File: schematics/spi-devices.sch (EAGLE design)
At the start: 13 parts, among them J1 DM3AT-SF-PEJM5, X1 87758-1016, X2 87758-0216

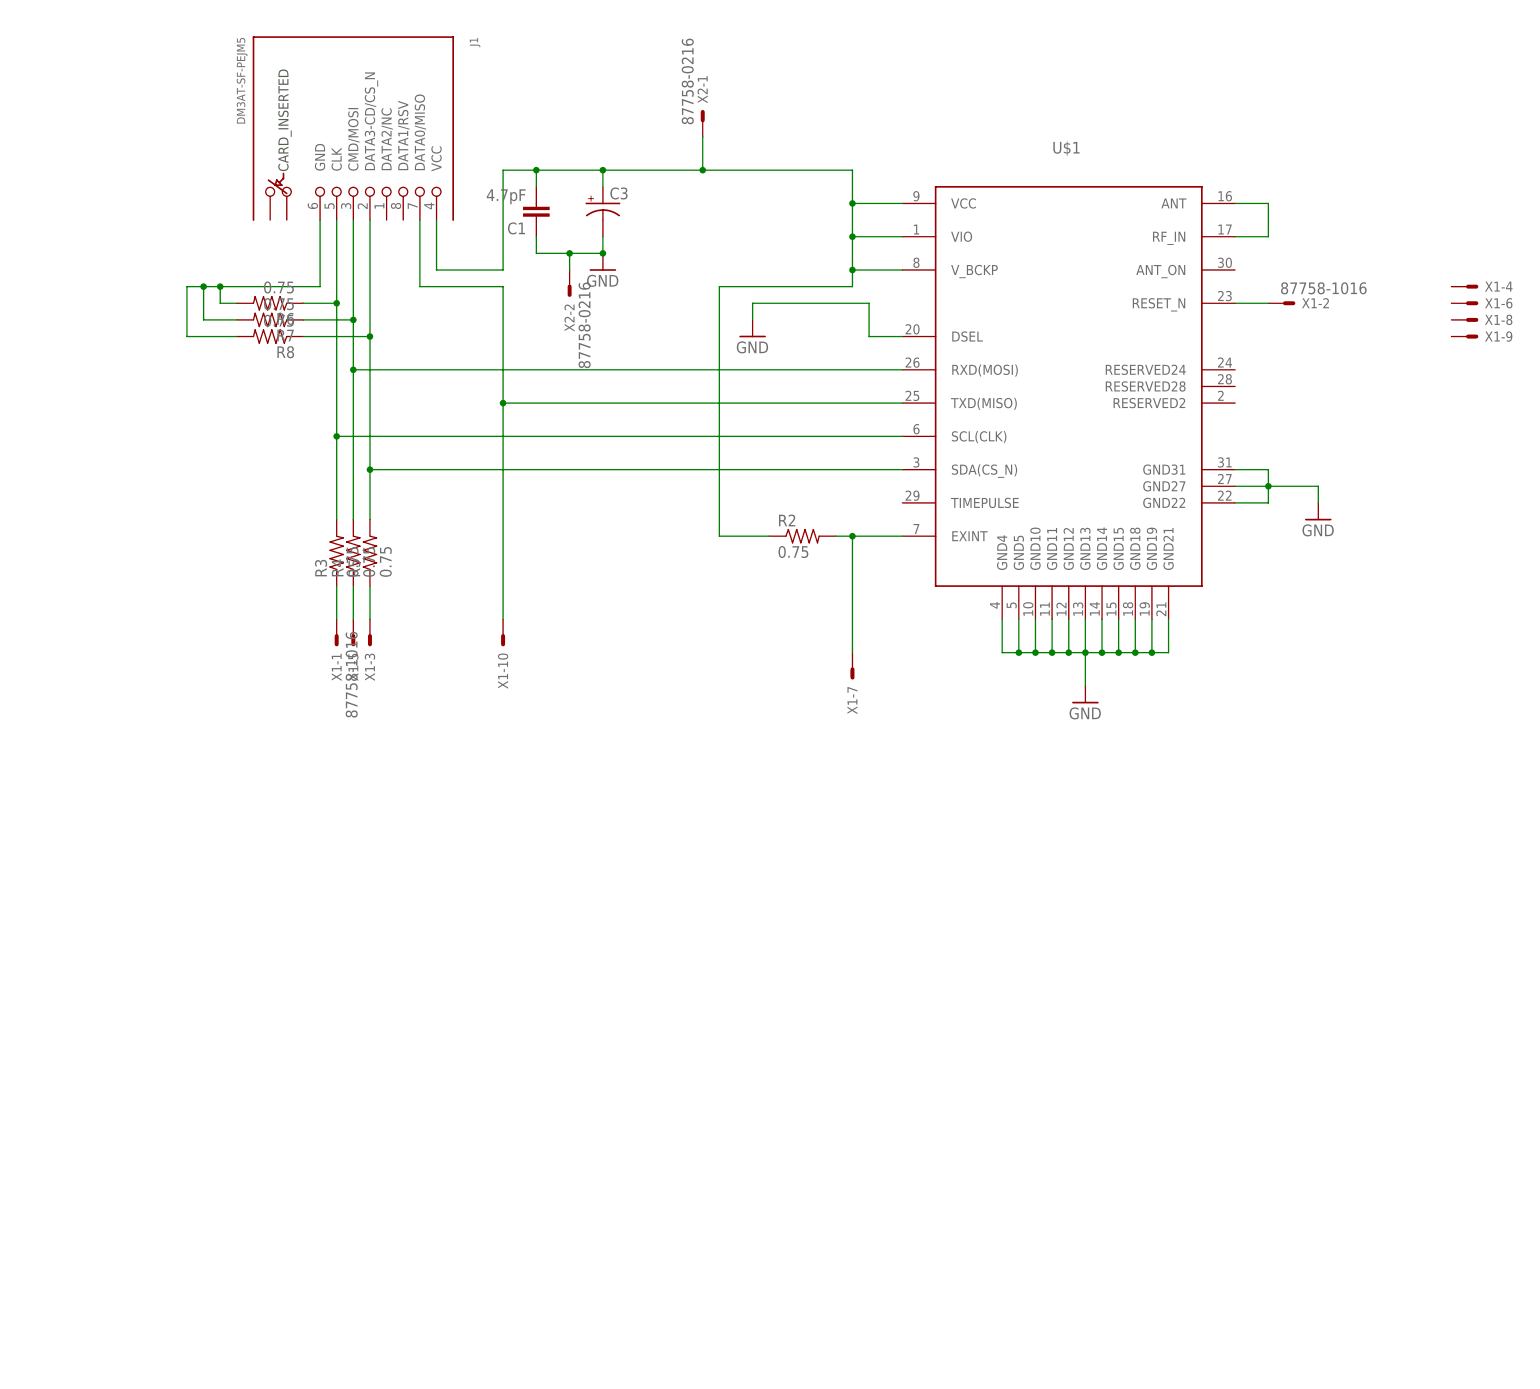
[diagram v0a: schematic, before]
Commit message: Платы, правки, накопленные изменения
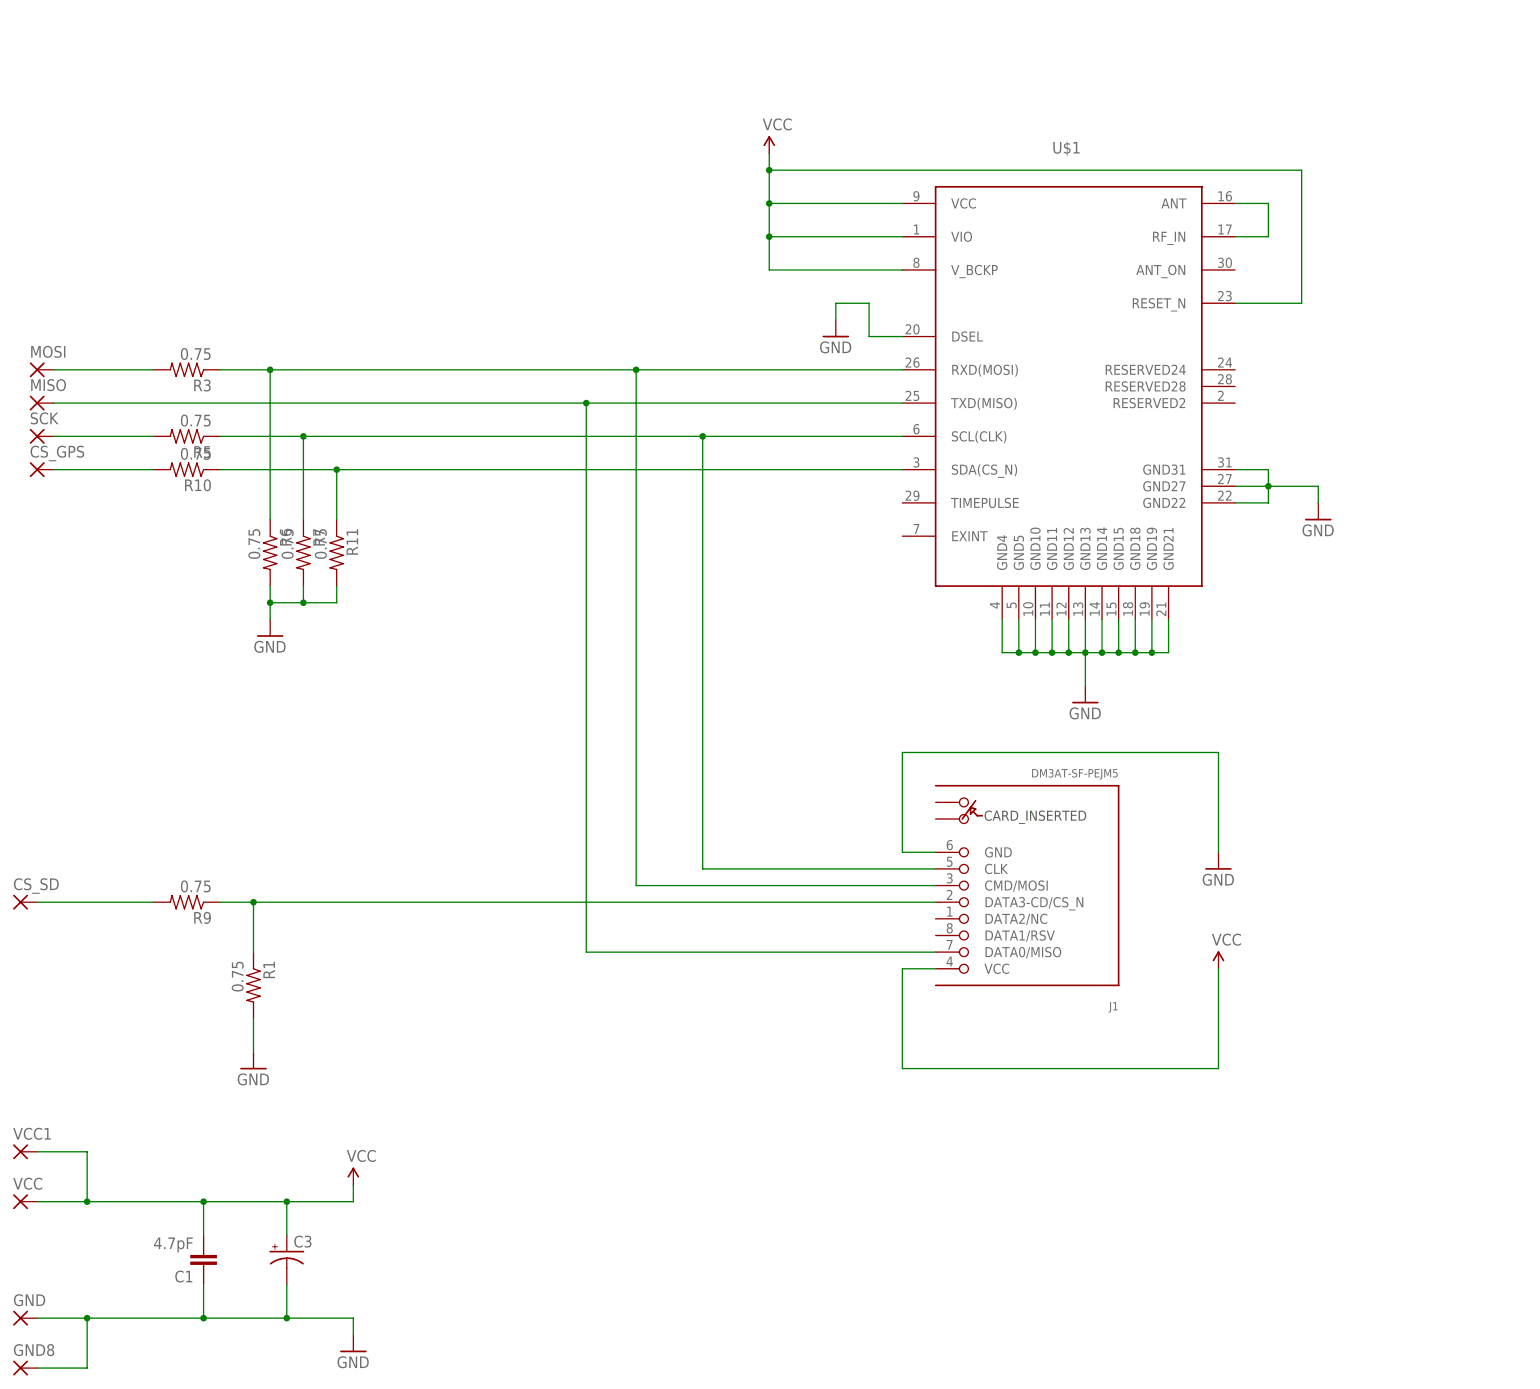
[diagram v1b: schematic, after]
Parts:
- removed R2, R4, R8: 0.75, SparkFun-Resistors:0.75OHM-1/4W-1%(0805)
- removed X1: 87758-1016, con-molex:87758-1016
- removed X2: 87758-0216, con-molex:87758-0216
- added CS_GPS, CS_SD, GND, GND8, MISO, MOSI, SCK, VCC, VCC1: (no value), wirepad:2,54/0,9
- added R1, R10, R11, R9: 0.75, SparkFun-Resistors:0.75OHM-1/4W-1%(0805)
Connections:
- net N$1 renamed RF
- removed net 3.3V: C1.2, C3.+, J1.VCC, R2.1, U$1.VCC, U$1.VIO, U$1.V_BCKP, X2-1.S
- removed net N$12: J1.CLK, R3.2, R6.1, U$1.SCL(CLK)
- removed net N$14: J1.DATA3-CD/CS_N, R5.2, R8.1, U$1.SDA(CS_N)
- removed net N$16: J1.CMD/MOSI, R4.2, R7.1, U$1.RXD(MOSI)
- removed net N$2: U$1.RESET_N, X1-2.S
- removed net N$3: R2.2, U$1.EXINT, X1-7.S
- removed net N$4: J1.DATA0/MISO, U$1.TXD(MISO), X1-10.S
- removed net N$5: R4.1, X1-5.S
- removed net N$6: R5.1, X1-3.S
- removed net N$7: J1.GND, R6.2, R7.2, R8.2
- removed net N$8: R3.1, X1-1.S
- new net CS_GPS: CS_GPS.P, R10.2
- new net CS_GPS_3.3: R10.1, R11.1, U$1.SDA(CS_N)
- new net CS_SD: CS_SD.P, R9.2
- new net CS_SD_3.3: J1.DATA3-CD/CS_N, R1.1, R9.1
- new net MISO: J1.DATA0/MISO, MISO.P, U$1.TXD(MISO)
- new net MOSI: MOSI.P, R3.2
- new net MOSI3.3: J1.CMD/MOSI, R3.1, R6.1, U$1.RXD(MOSI)
- new net SCK: R5.2, SCK.P
- new net SCK3.3: J1.CLK, R5.1, R7.1, U$1.SCL(CLK)
- new net VCC: C1.2, C3.+, J1.VCC, U$1.RESET_N, U$1.VCC, U$1.VIO, U$1.V_BCKP, VCC.P, VCC1.P
- net GND: now also GND.P, GND8.P, J1.GND, R1.2, R11.2, R6.2, R7.2; no longer X2-2.S
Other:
- moved on the sheet: C1, C3, J1, R3, R5, R6, R7
